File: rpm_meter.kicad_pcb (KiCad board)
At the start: 2 copper layers, 170.4 x 98.7 mm, 147 parts, among them IC1 SN74LV1T34DCKR, IC6 TPS566247DRLR, J1 Conn_01x01_Socket, J2 Conn_2Rows-05Pins, J3 Conn_01x01_Socket, J4 Conn_01x01_Socket, J5 Conn_01x01_Socket, J6 Conn_01x01_Socket, J7 Conn_01x01_Socket, Q1 BC846, Q14 BC846, Q15 BC846, Q16 BC846, SW1 RotaryEncoder_Switch_MP, U1 M24C02-RMN, U2 STM32C031C6Tx, U3 74LVC1G123, U4 TLV1117-33, Y1 8

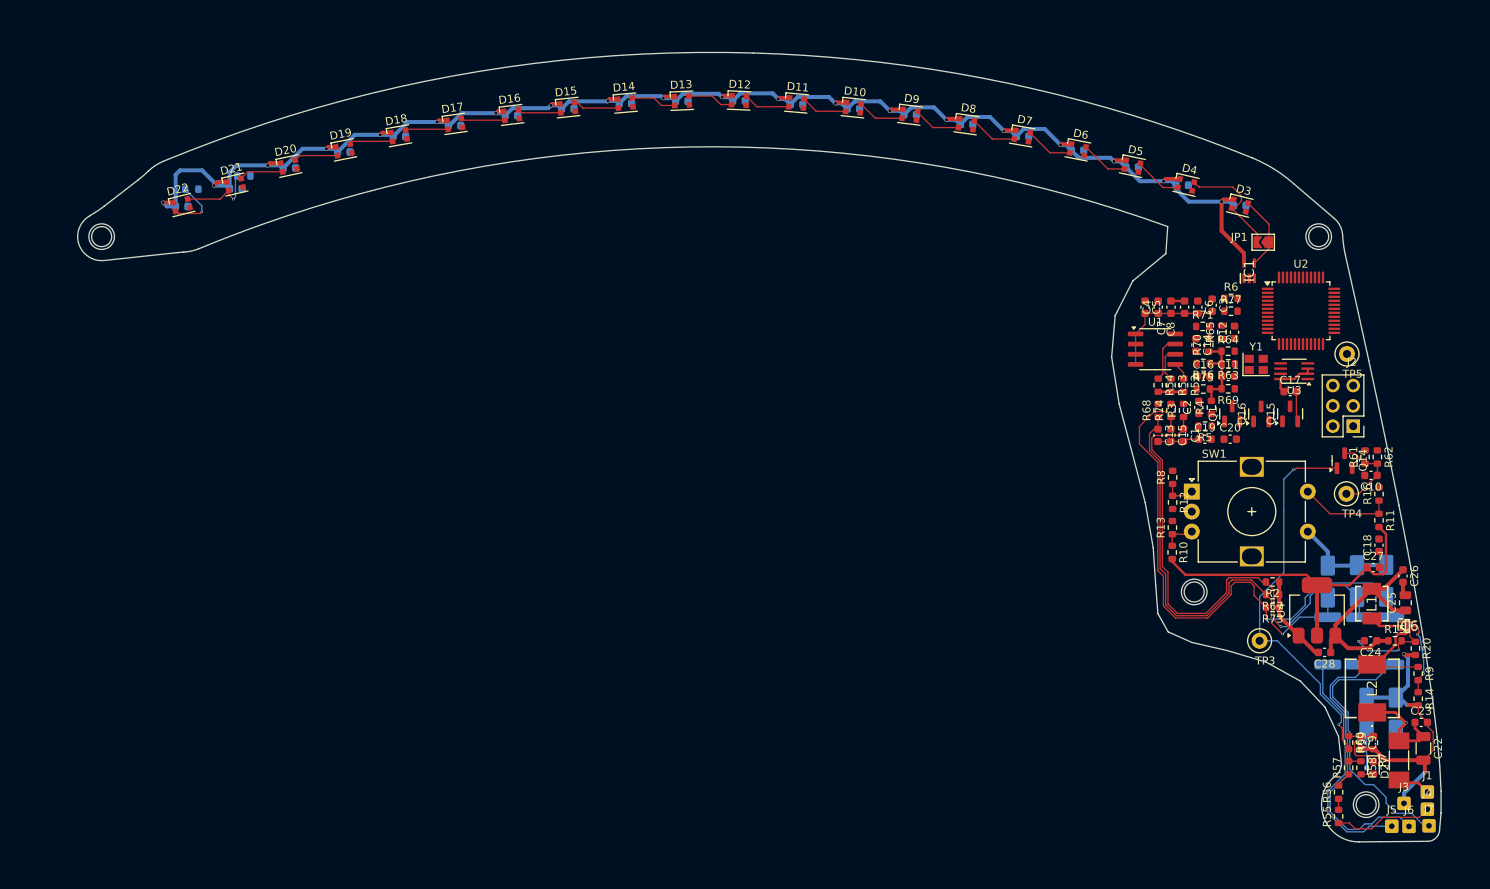
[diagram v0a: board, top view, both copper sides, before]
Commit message: routing2.0
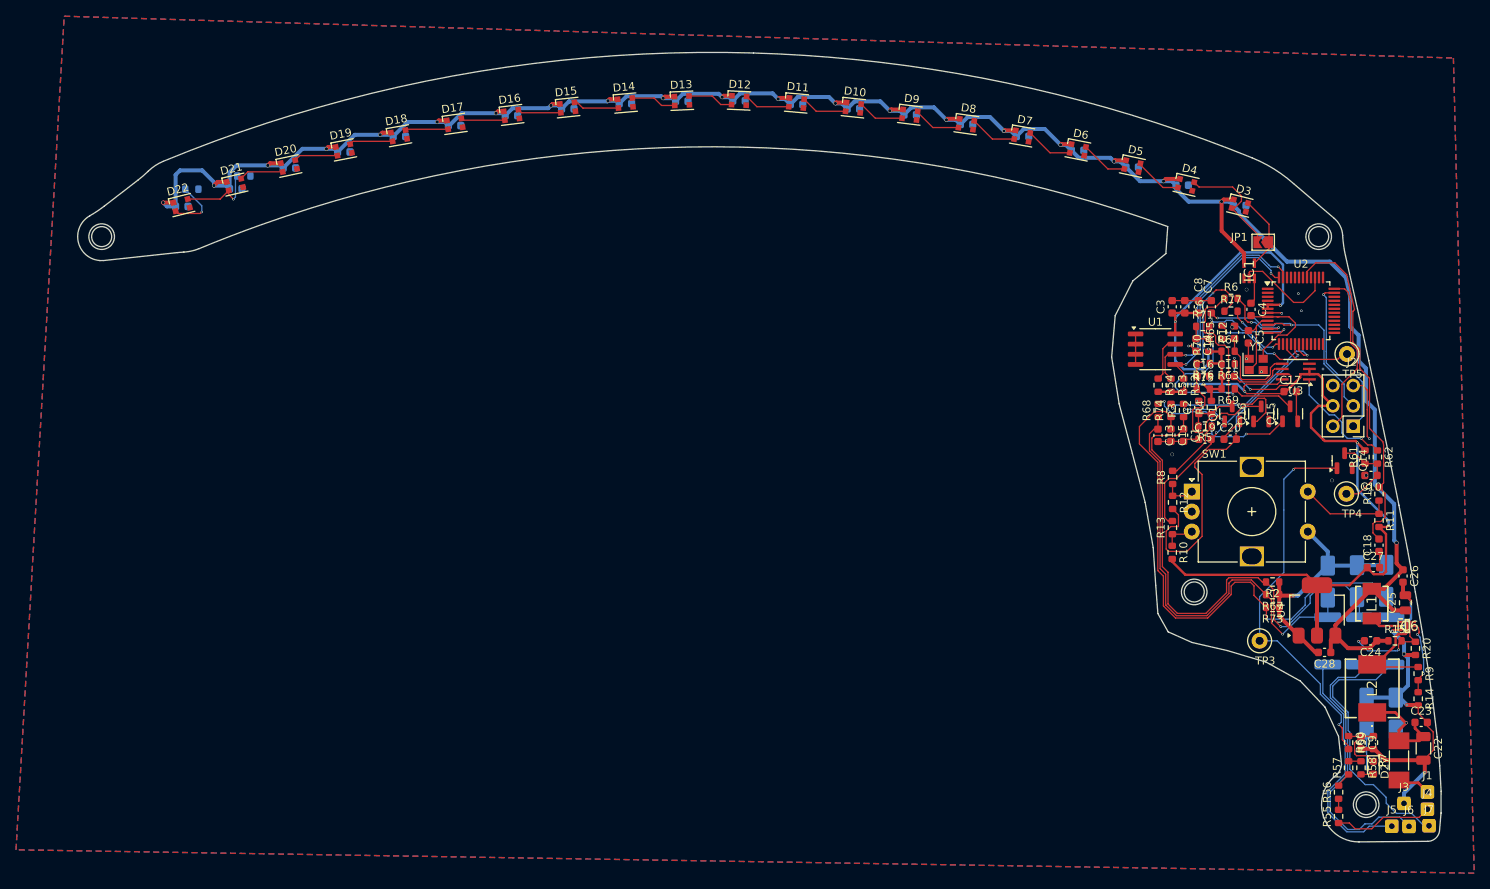
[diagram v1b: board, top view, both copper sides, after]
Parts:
- moved C5 13.4 mm to (206.5, 63.7)
- moved C4 11.6 mm to (206.8, 60.3), turned to -90 degrees
- moved C3 5.00 mm to (196.9, 60.0), turned to 90 degrees
- moved C7 3.43 mm to (200.2, 60.0), turned to -90 degrees
- moved C6 1.69 mm to (201.8, 60.0), turned to 90 degrees
- moved U3 0.20 mm to (212.4, 68.0)
- moved C8 0.06 mm to (198.5, 60.0), turned to -90 degrees
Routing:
- net +3.3V: track 63.7 -> 164.6 mm, vias 0 -> 8
- net +5V: track 225.3 -> 282.5 mm, vias 20 -> 21
- net /mcu/enc_p: track 0.00 -> 43.5 mm
- net /mcu/enc_a: track 0.00 -> 43.1 mm, vias 0 -> 2
- net Net-(Q16-C): track 0.00 -> 35.6 mm, vias 0 -> 2
- net /mcu/enc_b: track 0.00 -> 33.1 mm, vias 0 -> 2
- net GND: track 89.6 -> 121.2 mm, vias 3 -> 23
- net /mcu/NRST: track 0.00 -> 29.3 mm, vias 0 -> 2
- net Net-(Q15-C): track 0.00 -> 28.9 mm, vias 0 -> 2
- net /mcu/scl: track 4.40 -> 28.4 mm, vias 0 -> 2
- net Net-(Q1-C): track 0.00 -> 23.8 mm
- net /mcu/sda: track 2.20 -> 25.6 mm, vias 0 -> 2
- net /mcu/TMS: track 0.00 -> 21.6 mm, vias 0 -> 1
- net /mcu/rpm_signal_mcu: track 0.00 -> 20.5 mm, vias 0 -> 2
- net /mcu/TCK: track 0.00 -> 20.3 mm
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- added copper zone on B.Cu, net GND
- added copper zone on F.Cu, net GND
